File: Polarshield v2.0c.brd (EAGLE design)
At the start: 100 x 80 mm, 74 parts, among them IC1 MP2307, IC2 74541PW, IC3 74541PW, IC4 74541PW, IC5 74541PW, J1 1X2-3.5MM, U1 ARDUINO_MEGA_SHIELD, X1 2.1MMJACKTHM

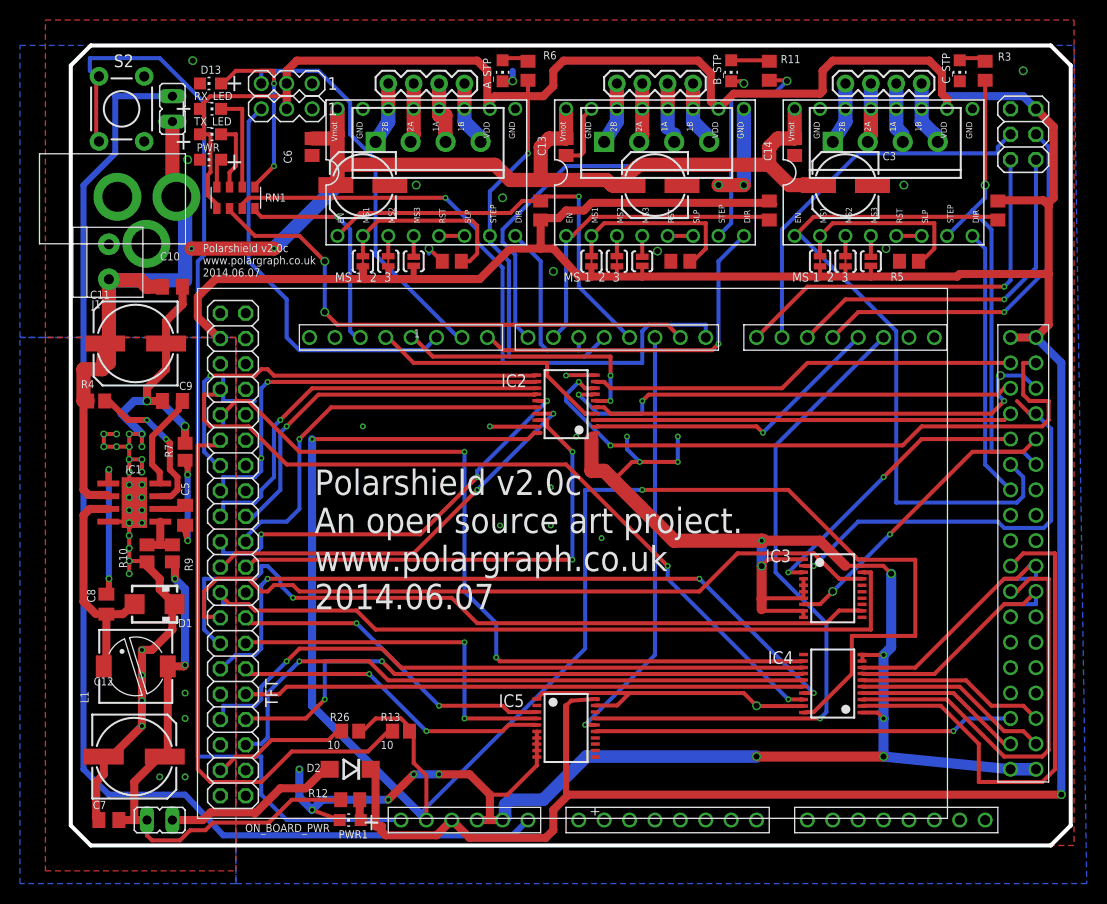
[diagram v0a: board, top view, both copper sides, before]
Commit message: v2c that has gone to the PCB makers last night.
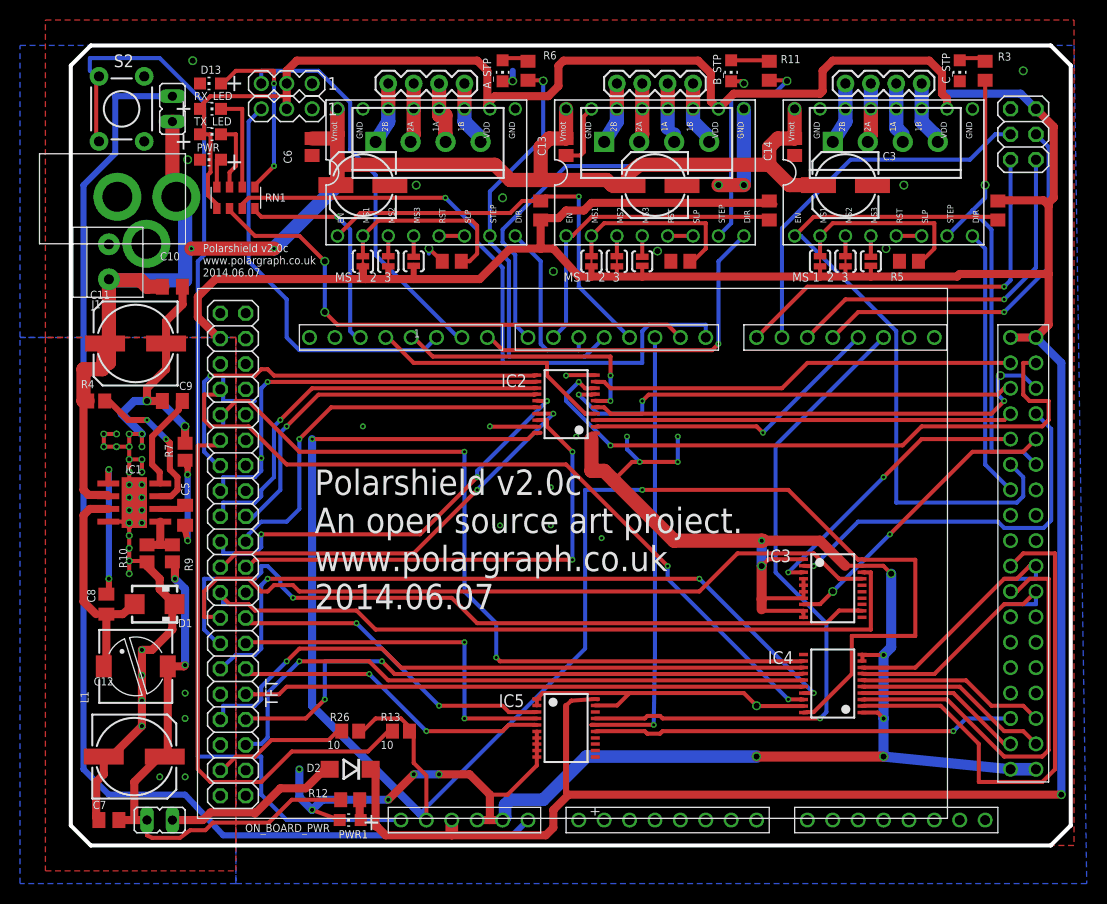
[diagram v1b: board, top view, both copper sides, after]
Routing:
- net D_PENIRQ: track 42.6 -> 45.3 mm
- net D27-TFT: track 40.9 -> 38.5 mm
- net A-STEP: track 40.3 -> 42.4 mm
- net GND: track 351.1 -> 351.8 mm
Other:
- board text added: "Polarshield v2.0c"
- board text removed: "Polarshield v2.0"
